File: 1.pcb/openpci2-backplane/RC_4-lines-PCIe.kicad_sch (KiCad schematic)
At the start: 32 parts, among them J2 PCIE-064-02-X-D-TH, J3 1-2199230-6, J4 525591652, U7 TPS563206DRLR, X1 39-28-1063

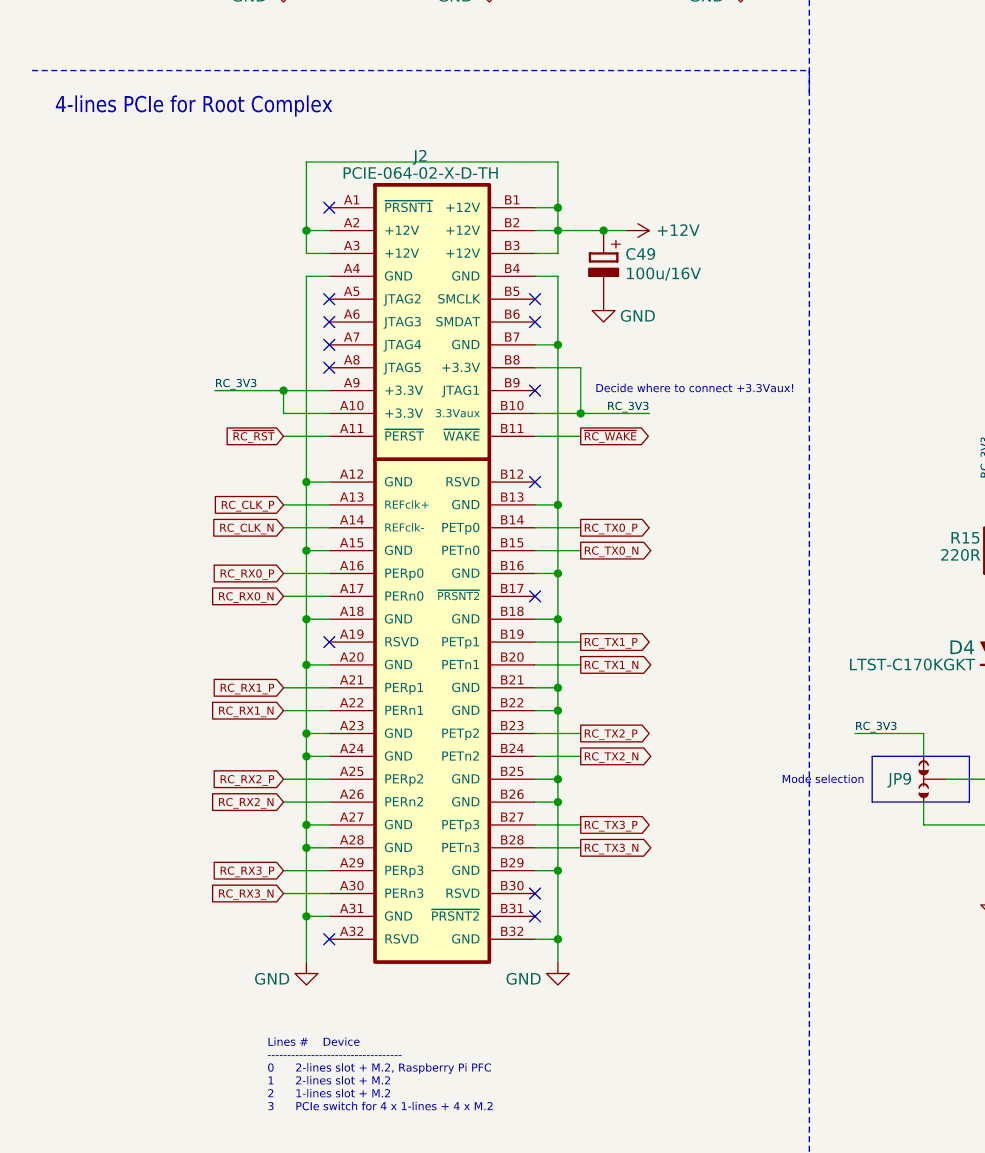
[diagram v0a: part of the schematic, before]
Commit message: PCIe connectors update
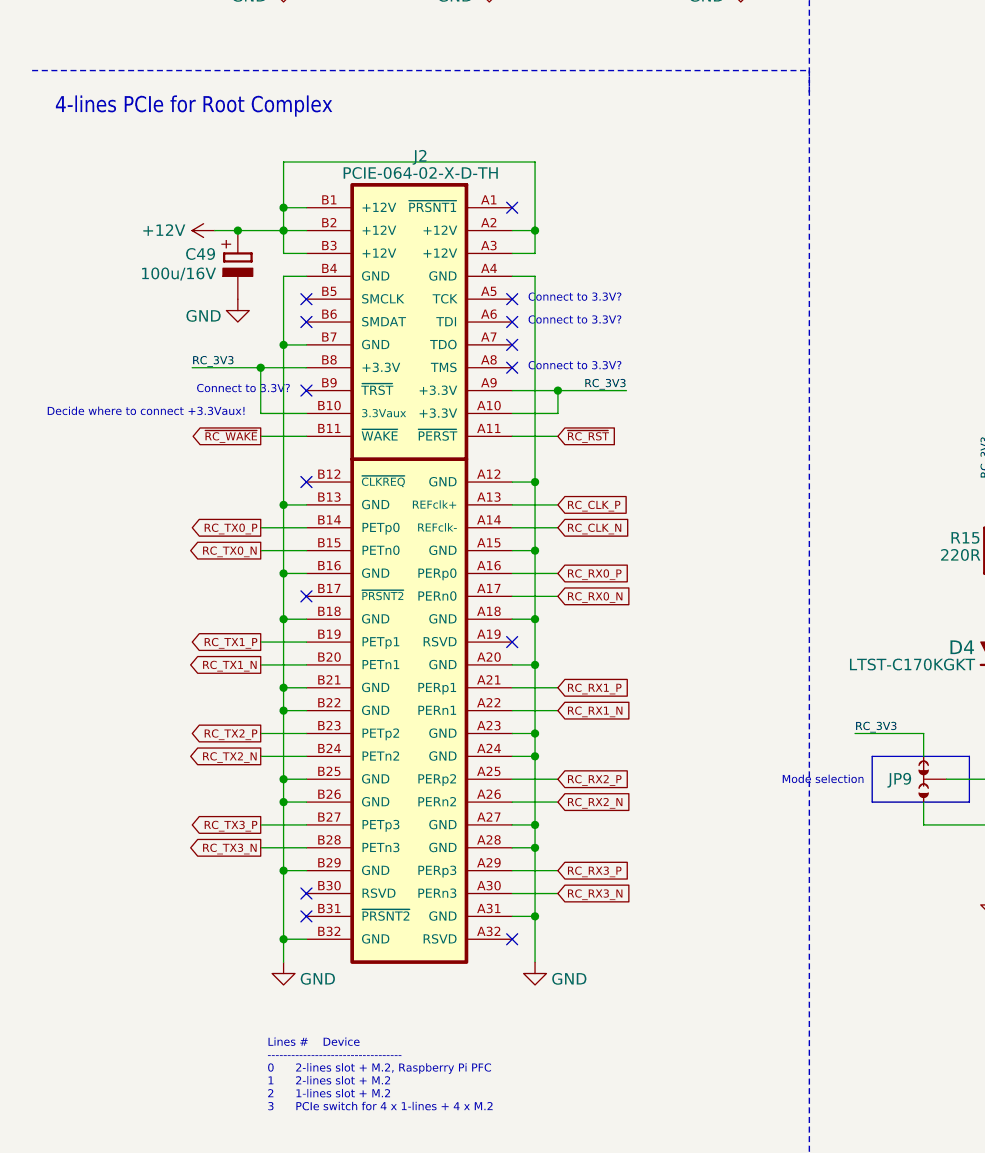
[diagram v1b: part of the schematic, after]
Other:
- note added: "Connect to 3.3V?"
- moved on the sheet: C49, J2
